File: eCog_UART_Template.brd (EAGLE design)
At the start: 48 x 28 mm, 1 part

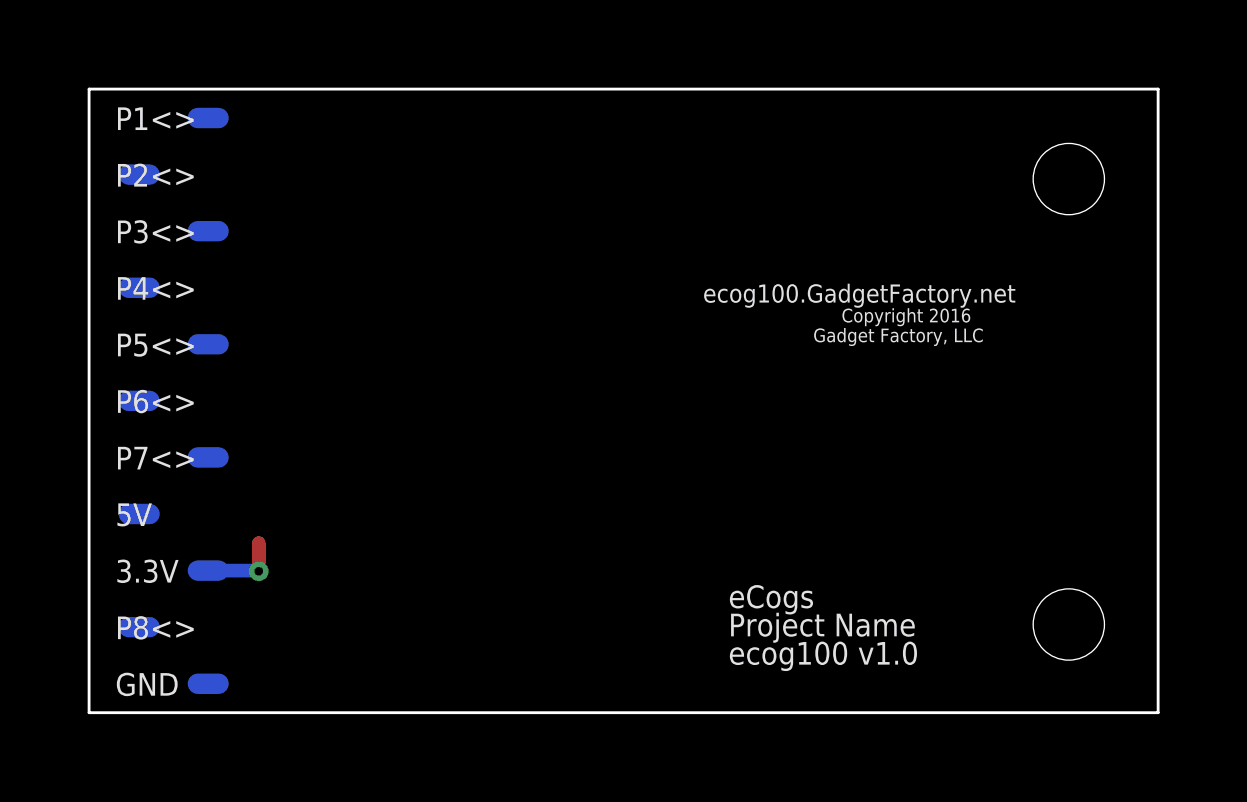
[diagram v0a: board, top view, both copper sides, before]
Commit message: Latest updated to V1.4
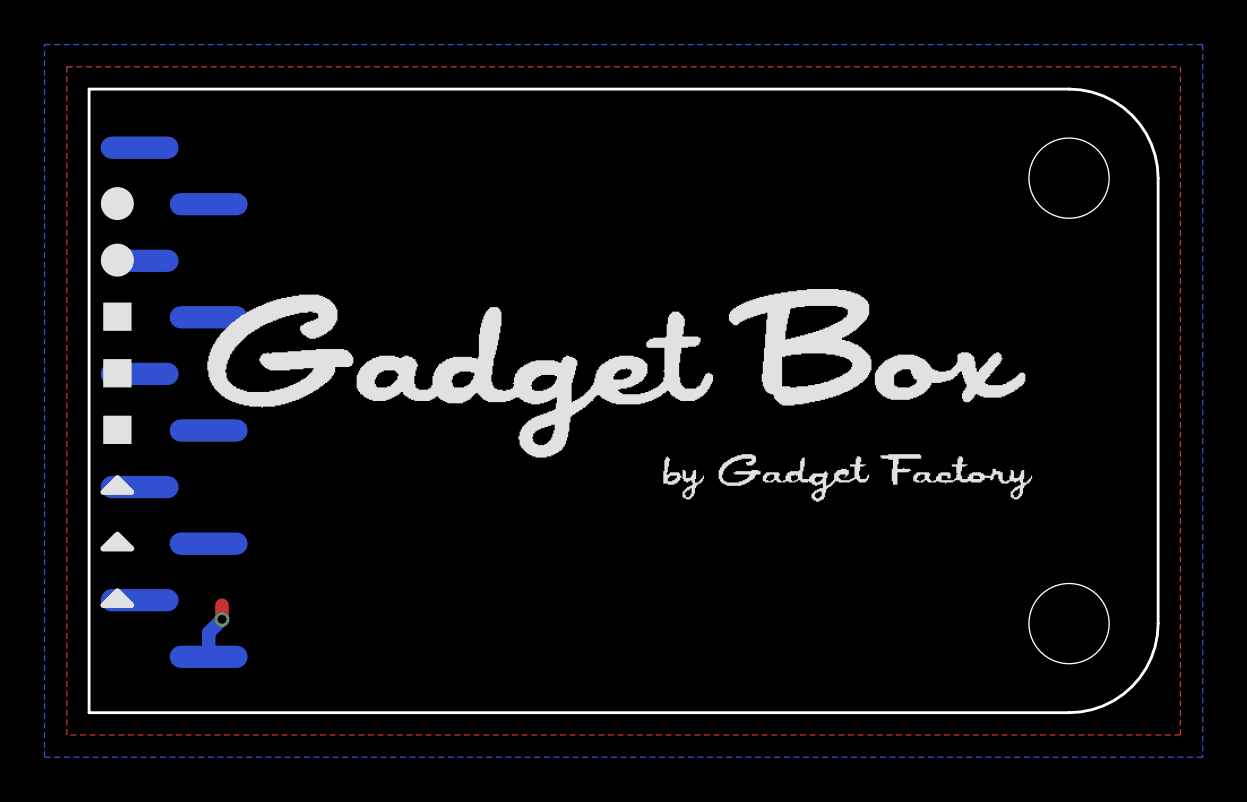
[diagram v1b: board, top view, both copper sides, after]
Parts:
- added U$1: (no value), GadgetFactory:GADGETBOX_TEXT
- added U$2, U$3: (no value), eCogs:LEGEND_DIO
- added U$4, U$5, U$6: (no value), eCogs:LEGEND_PWM
- added U$7, U$8, U$9: (no value), eCogs:LEGEND_ANALOG
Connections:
- net RX: now also ECOG.G1; no longer ECOG.2
- net TX: now also ECOG.G0; no longer ECOG.1
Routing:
- net 3V3: track 3.55 -> 2.56 mm
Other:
- outline, holes or cut-outs redrawn
- board text added: "G0<>"
- board text added: "G1<>"
- board text added: "G2<>"
- board text added: "G3<>"
- board text added: "G4<>"
- board text added: "G5<>"
- board text added: "G6<>"
- board text added: "G7<>"
- board text removed: "5V"
- board text removed: "P1<>"
- board text removed: "P2<>"
- board text removed: "P3<>"
- board text removed: "P4<>"
- board text removed: "P5<>"
- board text removed: "P6<>"
- board text removed: "P7<>"
- board text removed: "P8<>"
